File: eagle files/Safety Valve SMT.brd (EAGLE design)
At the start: 39.4 x 107.9 mm, 31 parts, among them IC1 TL072

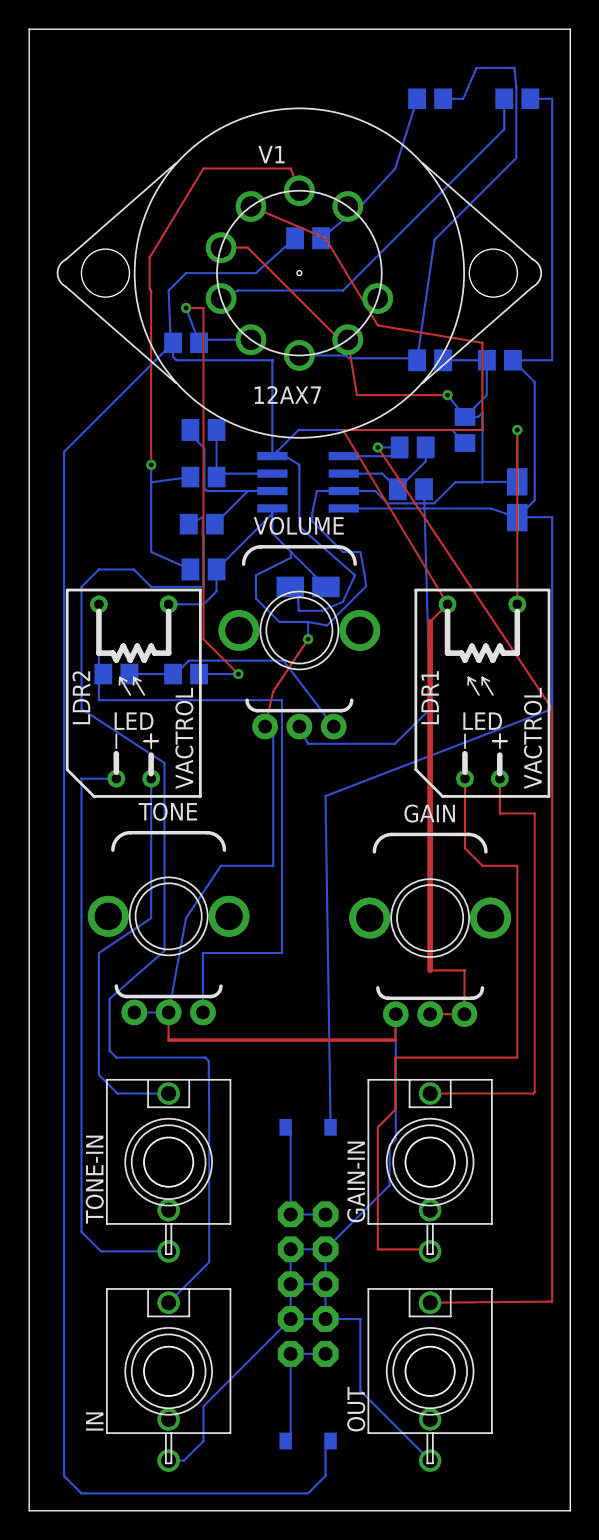
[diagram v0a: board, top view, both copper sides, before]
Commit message: enlarged all traces and added a ground plane
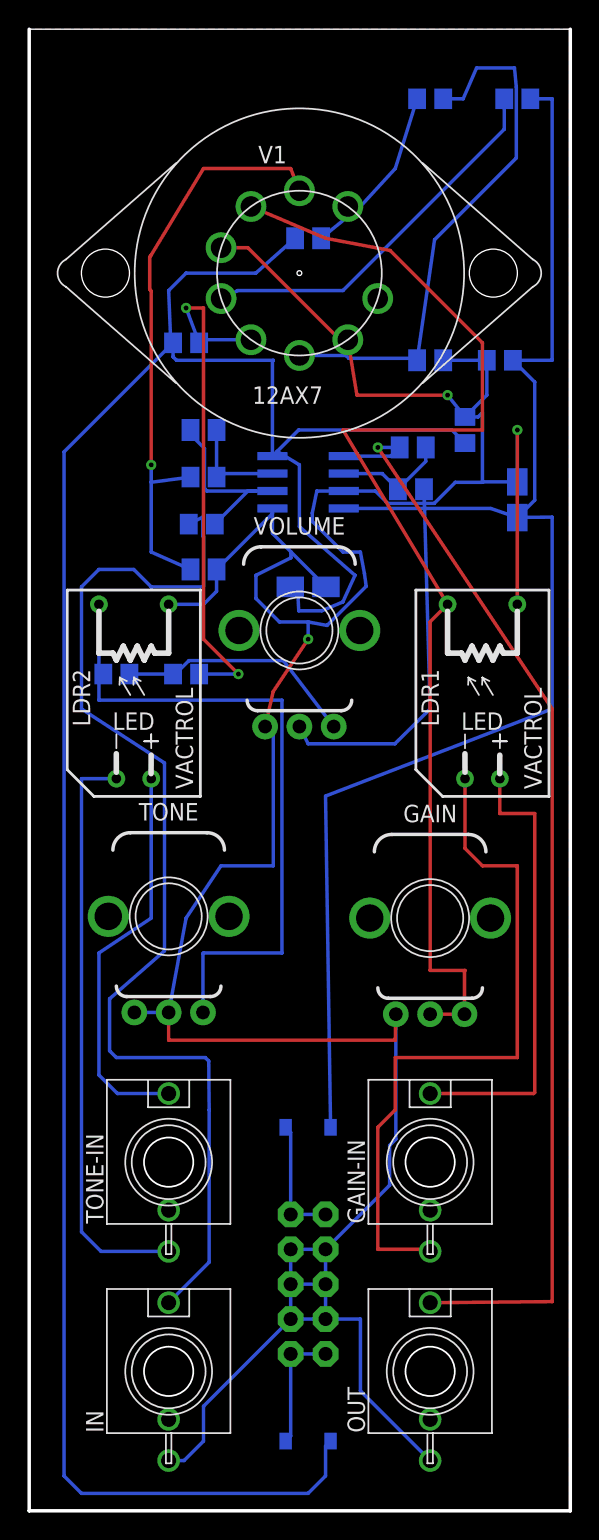
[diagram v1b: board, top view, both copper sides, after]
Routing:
- net N$1: track 88.4 -> 87.6 mm
- added copper zone on layer 1, net N$24

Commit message: Revert "enlarged all traces and added a ground plane"
This reverts commit 52d3814cfe846c563bf6933057c7568fe3819eec.
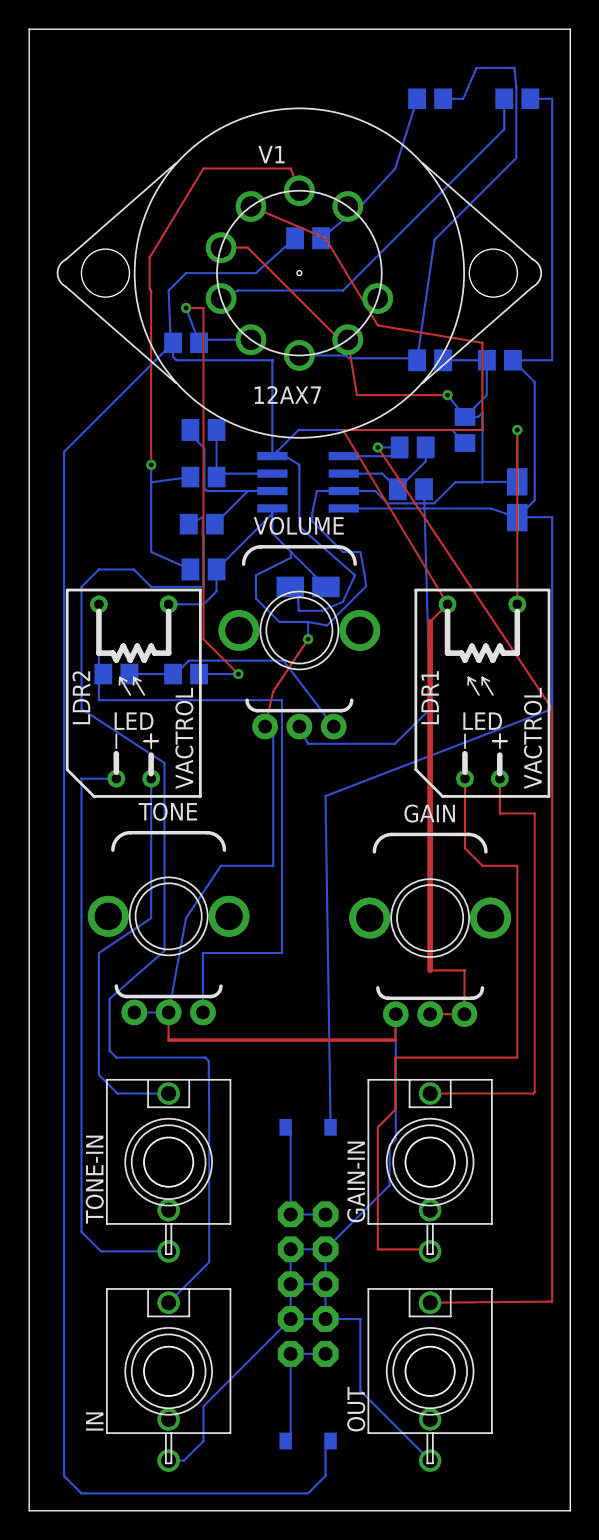
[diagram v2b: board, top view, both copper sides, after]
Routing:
- net N$1: track 87.6 -> 88.4 mm
- removed copper zone on layer 1, net N$24
